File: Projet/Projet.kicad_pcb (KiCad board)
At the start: 4 copper layers, 111 x 81 mm, 67 parts, among them J201 Conn_02x07_Odd_Even, J301 Moteur 1, J302 Moteur 1, J303 Conn_01x03, J401 optiqueGauche, J402 couleursDroit, J403 couleursGauche, J404 optiqueDroit, J405 tofGauche, J406 tofDroit, J501 alim batterie, J502 Conn_01x03_Female, SW201 SW_MEC_5E, U201 STM32G070RBT6, U301 ZXBM5210-S, U302 ZXBM5210-S, U501 AZ1117-5.0, U502 MIC5317-3.3, Y201 16 MHz

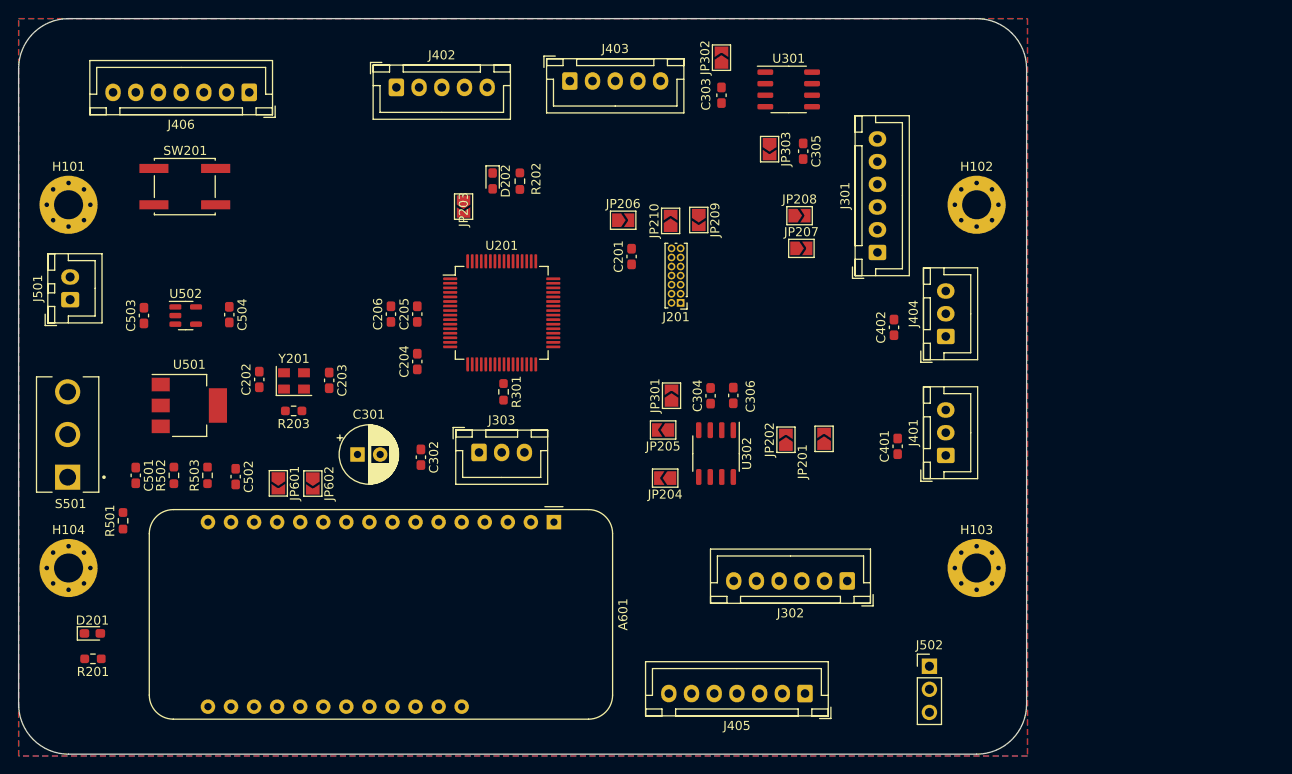
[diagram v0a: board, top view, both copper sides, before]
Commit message: Routing
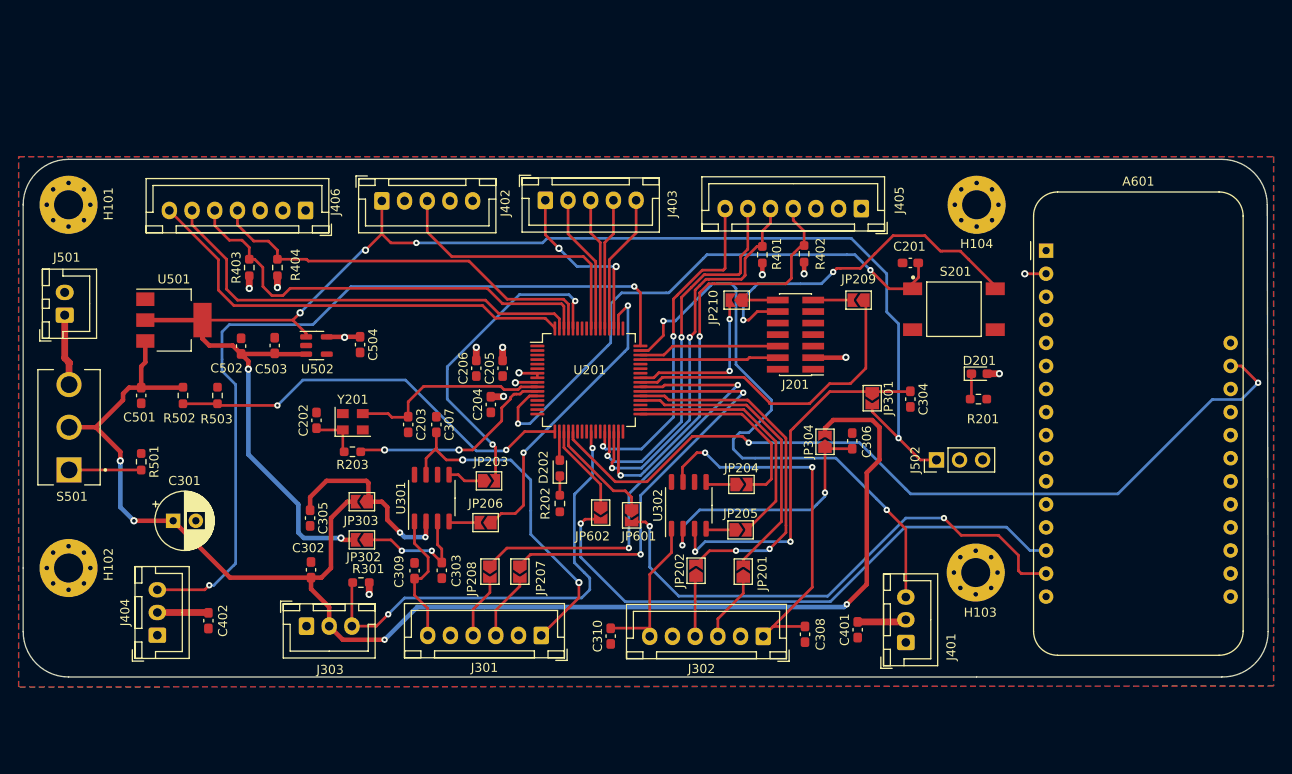
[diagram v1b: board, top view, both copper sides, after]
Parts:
- removed SW201: SW_MEC_5E, Button_Switch_SMD:SW_SPST_EVQQ2
- added C307: 1uF, Capacitor_SMD:C_0603_1608Metric_Pad1.08x0.95mm_HandSolder, F.Cu at (140.5, 124.2)
- added C308: 1uF, Capacitor_SMD:C_0603_1608Metric_Pad1.08x0.95mm_HandSolder, F.Cu at (181.1, 147.3)
- added C309: 1uF, Capacitor_SMD:C_0603_1608Metric_Pad1.08x0.95mm_HandSolder, F.Cu at (138.1, 140.3)
- added C310: 1uF, Capacitor_SMD:C_0603_1608Metric_Pad1.08x0.95mm_HandSolder, F.Cu at (159.7, 147.5)
- added JP304: SolderJumper_2_Open, Jumper:SolderJumper-2_P1.3mm_Open_TrianglePad1.0x1.5mm, F.Cu at (183.3, 126.1)
- added R401: 2.2k, Resistor_SMD:R_0603_1608Metric_Pad0.98x0.95mm_HandSolder, F.Cu at (176.4, 105.5)
- added R402: 2.2k, Resistor_SMD:R_0603_1608Metric_Pad0.98x0.95mm_HandSolder, F.Cu at (181.0, 105.4)
- added R403: 2.2k, Resistor_SMD:R_0603_1608Metric_Pad0.98x0.95mm_HandSolder, F.Cu at (119.9, 106.9)
- added R404: 2.2k, Resistor_SMD:R_0603_1608Metric_Pad0.98x0.95mm_HandSolder, F.Cu at (123.0, 106.9)
- added S201: 2-1437565-7, 2-1437565-7 (1):SW_2-1437565-7, F.Cu at (197.5, 111.5)
- C305, C306: value 100nF -> 10uF
- C502: value 10uF -> 22uF
- J201: footprint Connector_PinHeader_1.00mm:PinHeader_2x07_P1.00mm_Vertical -> Connector_PinHeader_1.27mm:PinHeader_2x07_P1.27mm_Vertical_SMD
- R201, R202: value 60R -> 1k
- R502: value 100k -> 200k
- R503: value 90k -> 100k
- moved H102 107.7 mm to (100.0, 140.0)
- moved H104 107.7 mm to (200.0, 100.0)
- moved D201 101.8 mm to (200.3, 118.6)
- moved R201 101.6 mm to (200.2, 121.4)
- moved J404 92.8 mm to (109.8, 147.4)
- moved C402 82.1 mm to (115.4, 145.8)
- moved C305 67.7 mm to (126.6, 134.5)
- moved JP302 66.2 mm to (132.3, 136.9), turned to 180 degrees
- moved A601 61.9 mm to (207.6, 105.0), turned to 0 degrees
- moved C303 60.7 mm to (141.1, 140.3)
- moved U301 59.7 mm to (140.0, 132.3), turned to 90 degrees
- moved JP303 59.4 mm to (132.3, 132.7), turned to 180 degrees
- moved J301 56.1 mm to (152.1, 147.4), turned to 180 degrees
- moved J405 53.8 mm to (187.3, 100.4)
- moved JP208 52.0 mm to (146.4, 140.4), turned to -90 degrees
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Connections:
- C201 pad 1: STLINK_NRST -> Net-(C201-Pad1)
- C306 pad 1: V+_batterie -> Net-(C306-Pad1)
- J402 pad 1: +3.3V -> +5V
- JP301 pad 2: +3.3V -> +5V
- JP302 pad 2: +3.3V -> +5V
- U201 pad 12: STLINK_NRST -> Net-(C201-Pad1)
- U201 pad 58: BAT_LED -> unconnected-(U201-Pad58)
- U201 pad 7: unconnected-(U201-Pad7) -> +3.3V
- U302 pad 2: V+_batterie -> Net-(C306-Pad1)
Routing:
- net +5V: track 0.00 -> 165.7 mm, vias 0 -> 6
- net V+_batterie: track 0.00 -> 159.7 mm, vias 0 -> 4
- net /Communication/ESP_EN: track 0.00 -> 91.8 mm, vias 0 -> 2
- net /STM32F070RB/OPTQ1: track 0.00 -> 90.2 mm, vias 0 -> 2
- net /STM32F070RB/OPTQ2: track 0.00 -> 66.6 mm, vias 0 -> 2
- net Net-(A601-Pad14): track 0.00 -> 63.8 mm, vias 0 -> 1
- net Net-(C201-Pad1): track 0.00 -> 62.8 mm, vias 0 -> 2
- net Net-(A601-Pad15): track 0.00 -> 58.8 mm, vias 0 -> 2
- net /Driver_Motor_SERVO/SERV_DATA: track 0.00 -> 51.7 mm, vias 0 -> 2
- net /STM32F070RB/TOF1_GPIO1: track 0.00 -> 49.9 mm
- net Net-(JP208-Pad1): track 0.00 -> 49.8 mm, vias 0 -> 2
- net /STM32F070RB/TOF2_SDA: track 0.00 -> 49.6 mm, vias 0 -> 2
- net /STM32F070RB/TOF1_XSHUT: track 0.00 -> 49.3 mm
- net /STM32F070RB/TOF1_SCL: track 0.00 -> 48.9 mm
- net Net-(JP207-Pad1): track 0.00 -> 47.7 mm, vias 0 -> 2
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- added copper zone on In2.Cu, net +3.3V
- added copper zone on B.Cu, net GND
- added copper zone on F.Cu, net GND
- added copper zone on In1.Cu, net GND
- removed copper zone on B.Cu, net (none)
- removed copper zone on F.Cu, net (none)
- removed copper zone on In1.Cu, net (none)
- removed copper zone on In2.Cu, net (none)
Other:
- board size 111 x 81 mm -> 137.1 x 57 mm
